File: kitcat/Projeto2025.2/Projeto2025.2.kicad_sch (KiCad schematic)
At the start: 23 parts, among them IC1 LA4182, J1 Conn_01x02, J2 Conn_01x02, J3 Conn_01x02, J4 Conn_01x02, J5 Conn_01x02

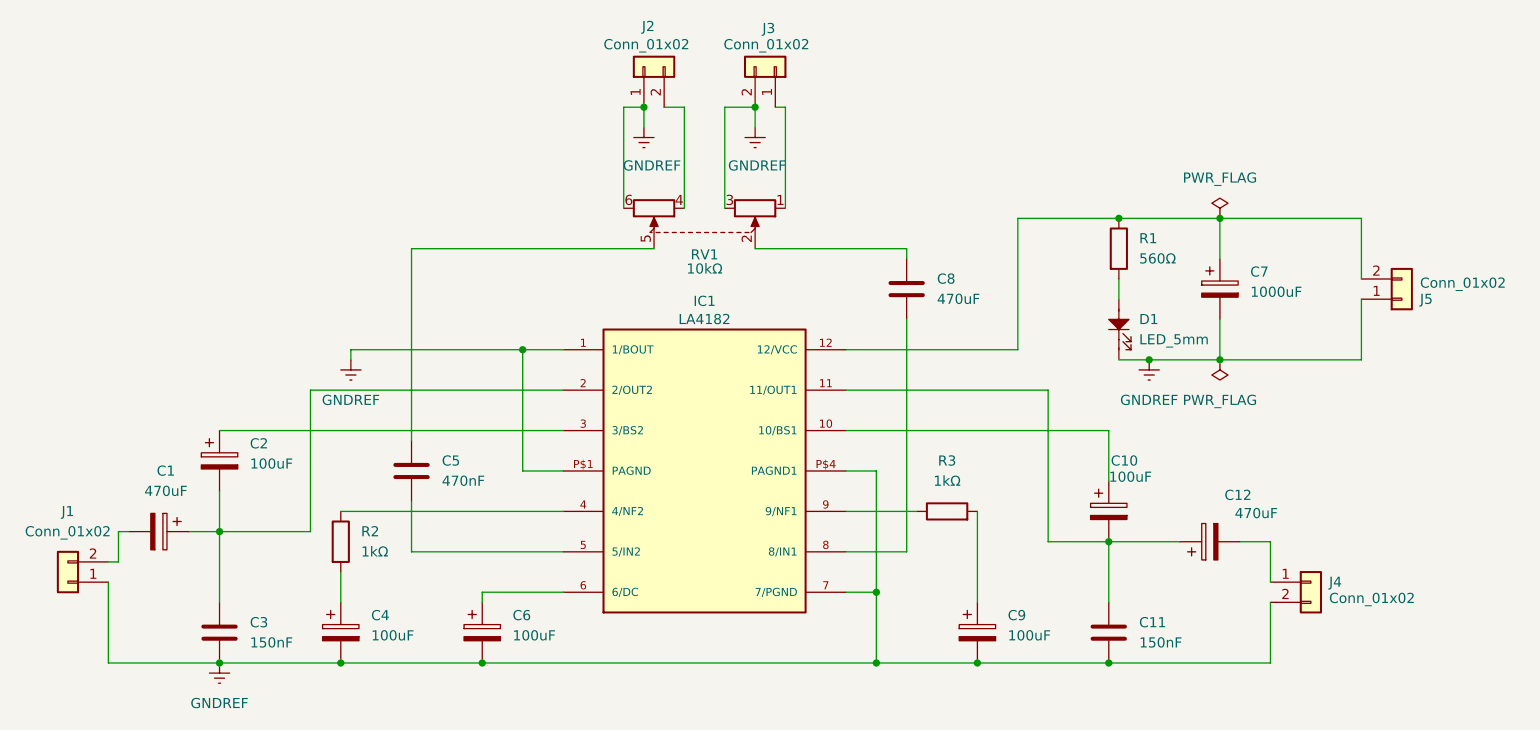
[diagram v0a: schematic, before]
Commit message: aaaaa
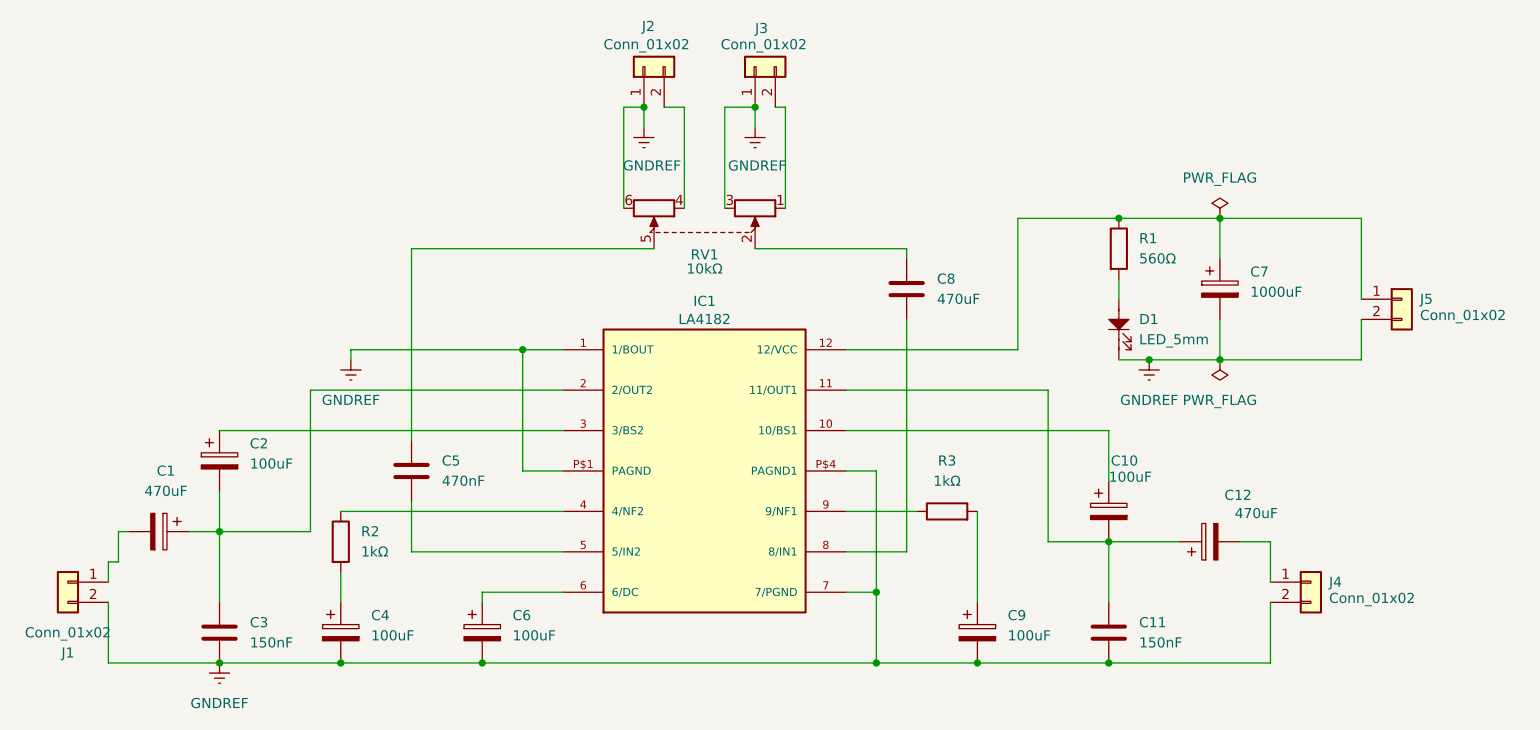
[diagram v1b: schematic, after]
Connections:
- net GNDREF: now also J1.2 (Pin_2), J3.1 (Pin_1), J5.2 (Pin_2); no longer J1.1 (Pin_1), J3.2 (Pin_2), J5.1 (Pin_1)
- net at C7.1, IC1.12 (12/VCC), R1.1: now also J5.1 (Pin_1); no longer J5.2 (Pin_2)
- net at C1.2: now also J1.1 (Pin_1); no longer J1.2 (Pin_2)
- net at RV1.1: now also J3.2 (Pin_2); no longer J3.1 (Pin_1)
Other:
- moved on the sheet: J1, J3, J5
